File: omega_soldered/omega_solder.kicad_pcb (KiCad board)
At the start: 2 copper layers, 200.8 x 58.9 mm, 64 parts, among them SW1 SW_Push, U1 ProMicro

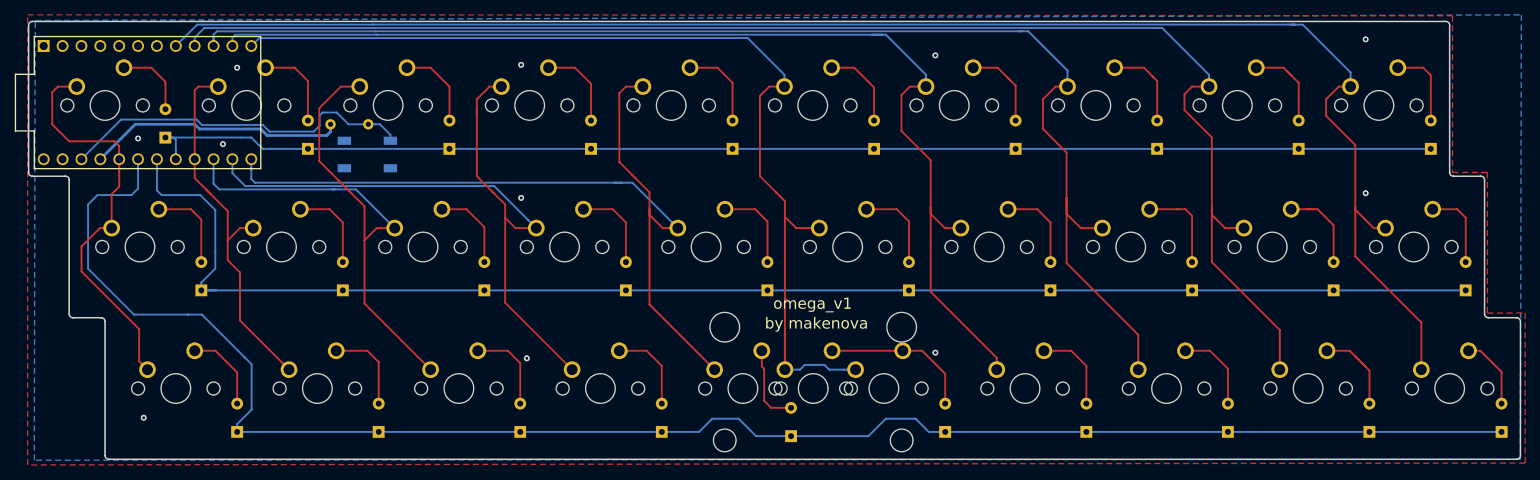
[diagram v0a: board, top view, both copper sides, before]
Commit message: work
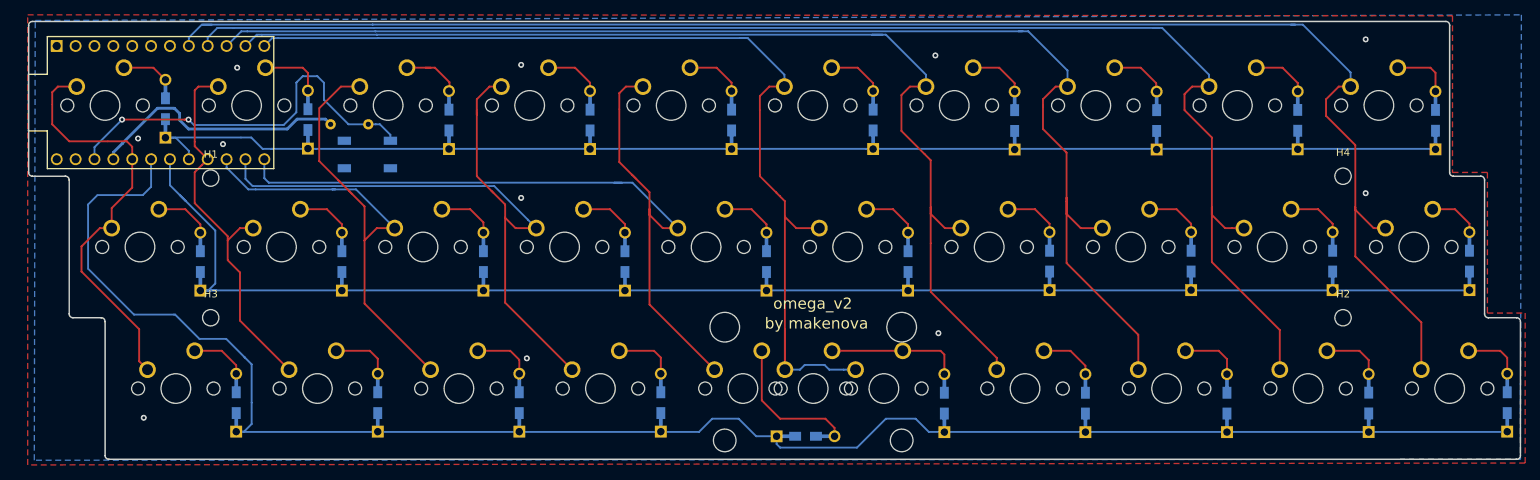
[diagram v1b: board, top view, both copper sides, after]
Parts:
- added H1: Hole, MountingHole:MountingHole_2.2mm_M2, F.Cu at (79.8, 60.7)
- added H2: Hole, MountingHole:MountingHole_2.2mm_M2, F.Cu at (232.2, 79.5)
- added H3: Hole, MountingHole:MountingHole_2.2mm_M2, F.Cu at (79.8, 79.5)
- added H4: Hole, MountingHole:MountingHole_2.2mm_M2, F.Cu at (232.2, 60.5)
- D1, D10, D11, D12, D13, D14, D15, D16, D17, D18, D19, D2, D20, D21, D22, D23, D24, D25, D26, D27, D28, D29, D3, D30, D4, D5, D6, D7, D8, D9: footprint Diode_THT:D_DO-35_SOD27_P3.81mm_Vertical_AnodeUp -> Keebio-Parts:Diode-Hybrid-Back; moved to F.Cu
- moved D30 4.01 mm to (254.3, 90.9), turned to 270 degrees
- moved D20 3.97 mm to (249.2, 71.9), turned to 270 degrees
- moved D17 3.94 mm to (192.7, 71.9), turned to 270 degrees
- moved D18 3.94 mm to (211.7, 71.9), turned to 270 degrees
- moved D19 3.94 mm to (230.8, 71.9), turned to 270 degrees
- moved D23 3.94 mm to (121.3, 90.9), turned to 270 degrees
- moved D21 3.94 mm to (83.2, 90.9), turned to 270 degrees
- moved D22 3.94 mm to (102.2, 90.9), turned to 270 degrees
- moved D24 3.94 mm to (140.3, 90.9), turned to 270 degrees
- moved D2 3.94 mm to (92.8, 52.8), turned to 270 degrees
- moved D10 3.89 mm to (244.6, 52.9), turned to 270 degrees
- moved D29 3.89 mm to (235.6, 91.0), turned to 270 degrees
- moved D11 3.88 mm to (78.4, 71.9), turned to 270 degrees
- moved D12 3.88 mm to (97.4, 71.9), turned to 270 degrees
- moved D13 3.88 mm to (116.5, 71.9), turned to 270 degrees
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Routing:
- net Net-(D25-Pad2): track 10.9 -> 19.1 mm
- net Net-(R1-Pad2): track 48.4 -> 54.3 mm, vias 0 -> 2
- net Net-(D29-Pad2): track 13.2 -> 8.02 mm
- net Net-(D19-Pad2): track 12.6 -> 7.53 mm
- net Net-(D18-Pad2): track 12.6 -> 7.53 mm
- net ROW2: track 231.5 -> 236.6 mm
- net Net-(D9-Pad2): track 12.5 -> 7.57 mm
- net Net-(D8-Pad2): track 12.1 -> 7.58 mm
- net Net-(D11-Pad2): track 12.0 -> 7.55 mm
- net Net-(D15-Pad2): track 11.9 -> 7.55 mm
- net Net-(D16-Pad2): track 11.9 -> 7.55 mm
- net Net-(D7-Pad2): track 11.9 -> 7.58 mm
- net Net-(D17-Pad2): track 11.8 -> 7.53 mm
- net Net-(D14-Pad2): track 11.8 -> 7.55 mm
- net Net-(D12-Pad2): track 11.8 -> 7.55 mm
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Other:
- board text added: "omega_v2"
- board text removed: "omega_v1"
